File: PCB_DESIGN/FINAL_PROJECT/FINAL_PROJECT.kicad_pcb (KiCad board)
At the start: 2 copper layers, 39 parts, among them J1 Conn_01x06_Pin, J2 Conn_01x02_Pin, J4 Barrel_Jack_Switch, J5 Conn_01x03, J6 XILINX_JTAG, J7 Conn_01x06_Pin, SW1 SW_SPST, U1 CA56-12CGKWA, U2 CA56-12CGKWA, U3 LFXP2-5E-5TN144, U4 LM317L, U5 LM7805, Y1 Oscillator

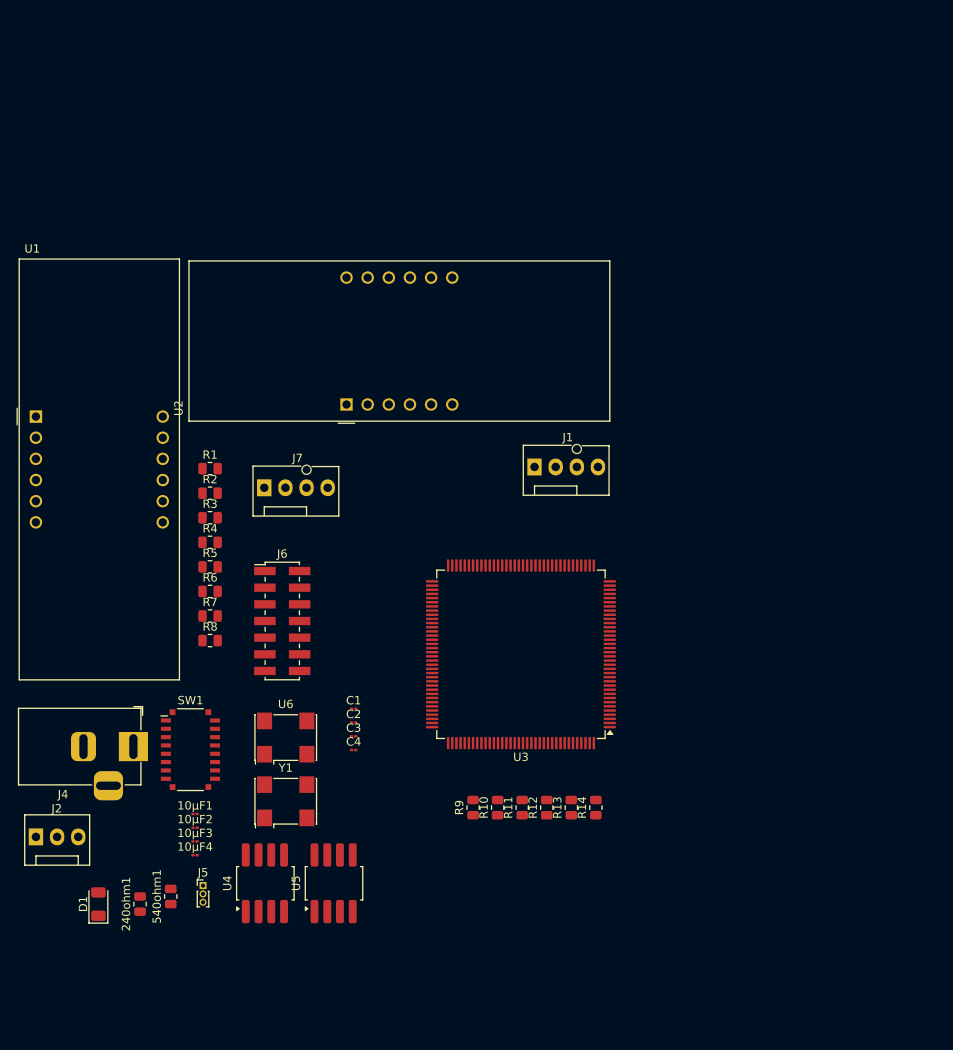
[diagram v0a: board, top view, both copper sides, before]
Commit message: Updated PCB
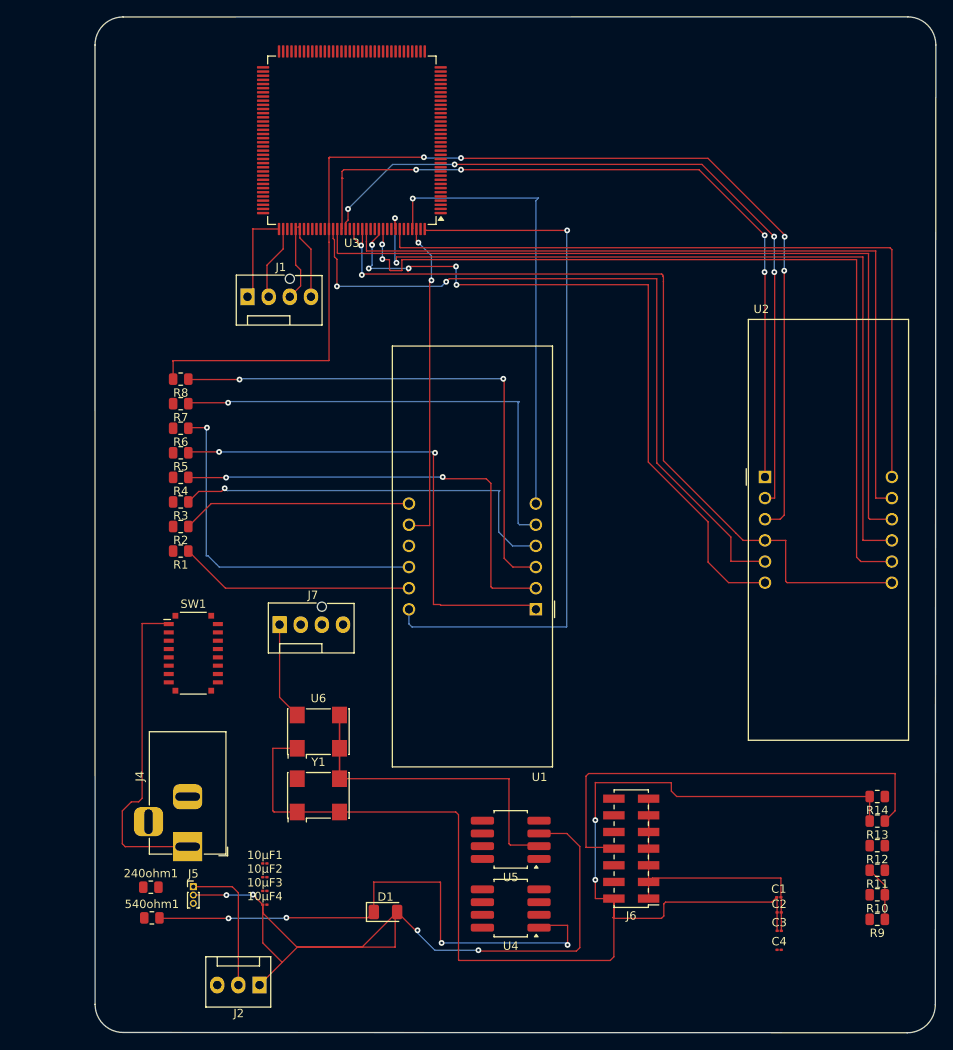
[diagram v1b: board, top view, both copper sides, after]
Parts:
- moved U3 65.0 mm to (157.9, 38.3)
- moved U1 64.4 mm to (180.0, 94.6), turned to 180 degrees
- moved C4 56.4 mm to (209.3, 135.5)
- moved C3 56.2 mm to (209.3, 133.2)
- moved C2 56.0 mm to (209.3, 131.0)
- moved C1 55.9 mm to (209.2, 129.2)
- moved U2 51.0 mm to (207.6, 78.7), turned to 0 degrees
- moved R9 50.4 mm to (221.0, 131.8), turned to 180 degrees
- moved J6 50.0 mm to (191.5, 123.3), turned to 180 degrees
- moved R10 46.8 mm to (221.0, 128.9), turned to 180 degrees
- moved R11 43.3 mm to (221.0, 125.9), turned to 180 degrees
- moved J1 40.1 mm to (145.4, 57.1)
- moved R12 40.0 mm to (221.0, 123.0), turned to 180 degrees
- moved R13 36.8 mm to (221.0, 120.0), turned to 180 degrees
- moved D1 34.5 mm to (162.0, 130.9), turned to 0 degrees
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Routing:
- net +3.3V: track 0.00 -> 164.2 mm, vias 0 -> 2
- net Net-(U2-DPX): track 0.00 -> 140.1 mm, vias 0 -> 4
- net Net-(U2-CA3): track 0.00 -> 103.4 mm, vias 0 -> 2
- net Net-(U2-b): track 0.00 -> 102.9 mm, vias 0 -> 2
- net /powersupply/5v: track 0.00 -> 101.8 mm, vias 0 -> 4
- net Net-(U2-f): track 0.00 -> 101.4 mm
- net Net-(U2-CA2): track 0.00 -> 101.0 mm, vias 0 -> 2
- net Net-(U2-a): track 0.00 -> 95.5 mm
- net Net-(U2-d): track 0.00 -> 92.1 mm, vias 0 -> 4
- net Net-(U2-e): track 0.00 -> 90.4 mm, vias 0 -> 4
- net Net-(U2-CA1): track 0.00 -> 88.7 mm
- net Net-(U2-g): track 0.00 -> 87.6 mm, vias 0 -> 2
- net Net-(U2-CA4): track 0.00 -> 86.4 mm, vias 0 -> 5
- net Net-(U1-CA1): track 0.00 -> 85.7 mm, vias 0 -> 1
- net GND: track 0.00 -> 84.3 mm
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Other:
- board outline added: 101 x 122 mm
